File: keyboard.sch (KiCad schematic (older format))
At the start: 74 parts, among them IC1 ATMEGA32U4, J1 MINI, P1 MISO, P10 ROW4, P18 LR1, P19 LR2, P2 Vcc, P20 LR3, P200 GND, P201 GND, P202 GND, P203 GND, P21 LR4, P23 LC1, P24 LC2, P25 LC3, P26 LC4, P27 LC5, P28 LC6, P29 LC7, P3 SCK, P30 LC8, P31 LC9, P32 LC10, P33 LC11, P34 LC12, P35 LGND, P36 LVcc, P37 Vcc, P38 GPIO0, P39 GPIO1, P4 MOSI, P40 GPIO2, P41 GPIO3, P42 GPIO4(SS), P43 GPIO5(SCK), P44 GPIO6(MOSI), P45 GPIO7(SCL), P46 GPIO8(SDA), P47 GND, P5 RES, P6 GND, P7 ROW1, P8 ROW2, P9 ROW3, X1 CRYSTAL

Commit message: Rebuild the project using latest kicad
Rebuild the project using latest kicad, leaving eschematic and pcb
unfinished
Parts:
- removed C4, C5, C6, C7: 100n, symbol C
- removed C8: 1u, symbol C
- removed DF3, DW1, DW2, DW3, DW4: LED, symbol LED
- removed H1, H2, H3, H4, H5: HOLE, ~, symbol ANYTHING
- removed J1: MINI, symbol USBMINI_B05
- removed P1: MISO, symbol CONN_1
- removed P10: ROW4, symbol CONN_1
- removed P18: LR1, symbol CONN_1
- removed P19: LR2, symbol CONN_1
- removed P2, P37: Vcc, symbol CONN_1
- removed P20: LR3, symbol CONN_1
- removed P200, P201, P202, P203, P47, P6: GND, symbol CONN_1
- removed P21: LR4, symbol CONN_1
- removed P23: LC1, symbol CONN_1
- removed P24: LC2, symbol CONN_1
- removed P25: LC3, symbol CONN_1
- removed P26: LC4, symbol CONN_1
- removed P27: LC5, symbol CONN_1
- removed P28: LC6, symbol CONN_1
- removed P29: LC7, symbol CONN_1
- removed P3: SCK, symbol CONN_1
- removed P30: LC8, symbol CONN_1
- removed P31: LC9, symbol CONN_1
- removed P32: LC10, symbol CONN_1
- removed P33: LC11, symbol CONN_1
- removed P34: LC12, symbol CONN_1
- removed P35: LGND, symbol CONN_1
- removed P36: LVcc, symbol CONN_1
- removed P38: GPIO0, symbol CONN_1
- removed P39: GPIO1, symbol CONN_1
- removed P4: MOSI, symbol CONN_1
- removed P40: GPIO2, symbol CONN_1
- removed P41: GPIO3, symbol CONN_1
- removed P42: GPIO4(SS), symbol CONN_1
- removed P43: GPIO5(SCK), symbol CONN_1
- removed P44: GPIO6(MOSI), symbol CONN_1
- removed P45: GPIO7(SCL), symbol CONN_1
- removed P46: GPIO8(SDA), symbol CONN_1
- removed P5: RES, symbol CONN_1
- removed P7: ROW1, symbol CONN_1
- removed P8: ROW2, symbol CONN_1
- removed P9: ROW3, symbol CONN_1
- removed R12, RW1, RW2, RW3, RW4: R, symbol R
- removed R3: 10k, symbol R
- removed X1: CRYSTAL, symbol CRYSTAL
- added J?: USBMINI_B05, symbol USBMINI_B05
- added R?: R, symbol R
- added X?: CRYSTAL, symbol CRYSTAL
- C1, C2: value 22p -> 22pF; Product CL21C220JBANNNC -> (none); Supplier TME -> (none); Supplier Symbol CL21C220JBANNNC -> (none); Vendor Samsung -> (none)
- C3: value 1u -> 1uF; Product CL21B105KAFNNNE -> (none); Supplier TME -> (none); Supplier Symbol CL21B105KAFNNNE -> (none); Vendor Samsung -> (none)
- IC1: Product ATmega32U4-AU -> (none); Supplier DigiKey -> (none); Supplier Symbol ATMEGA32U4-AU-ND -> (none); Vendor Atmel -> (none)
- R1, R2: value 22 -> 22R; Product CRCW080522R0JNTABC -> (none); Supplier TME -> (none); Supplier Symbol CRCW080522R0JNTABC -> (none); Vendor Vishay -> (none)
- R5: value 10k -> 10K; Product CRCW080510K0JNTABC -> (none); Supplier TME -> (none); Supplier Symbol CRCW080510K0JNTABC -> (none); Vendor Vishay -> (none)
- S0: Product TACTB-64K-F -> (none); Supplier TME -> (none); Supplier Symbol TACTB-64K-F -> (none); Vendor Ninigi -> (none)
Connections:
- net labels removed: D+, D-, GPIO0, GPIO1, GPIO2, GPIO3, GPIO4, GPIO5, GPIO6, GPIO7, GPIO8, MISO, MOSI, SCK, SCL, SDA, SS, caps, col1, col10, col11, col2, col3, col4, col5, col6, col7, col8, col9, row1, row2, row3, row4, ~RES~
- wire segments 168 -> 46
- no-connect marks 4 -> 2
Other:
- note removed: "Expansion\nconnector \n(right)"
- note removed: "FN LED\n"
- note removed: "Ground Pins"
- note removed: "ISP Pins"
- note removed: "LED Matrix\n(top)"
- note removed: "Mounting\nHoles"
- note removed: "PWM"
- note removed: "SW01 LED (ESCAPE)\n"
- note removed: "WASD Cluster LEDs\n"

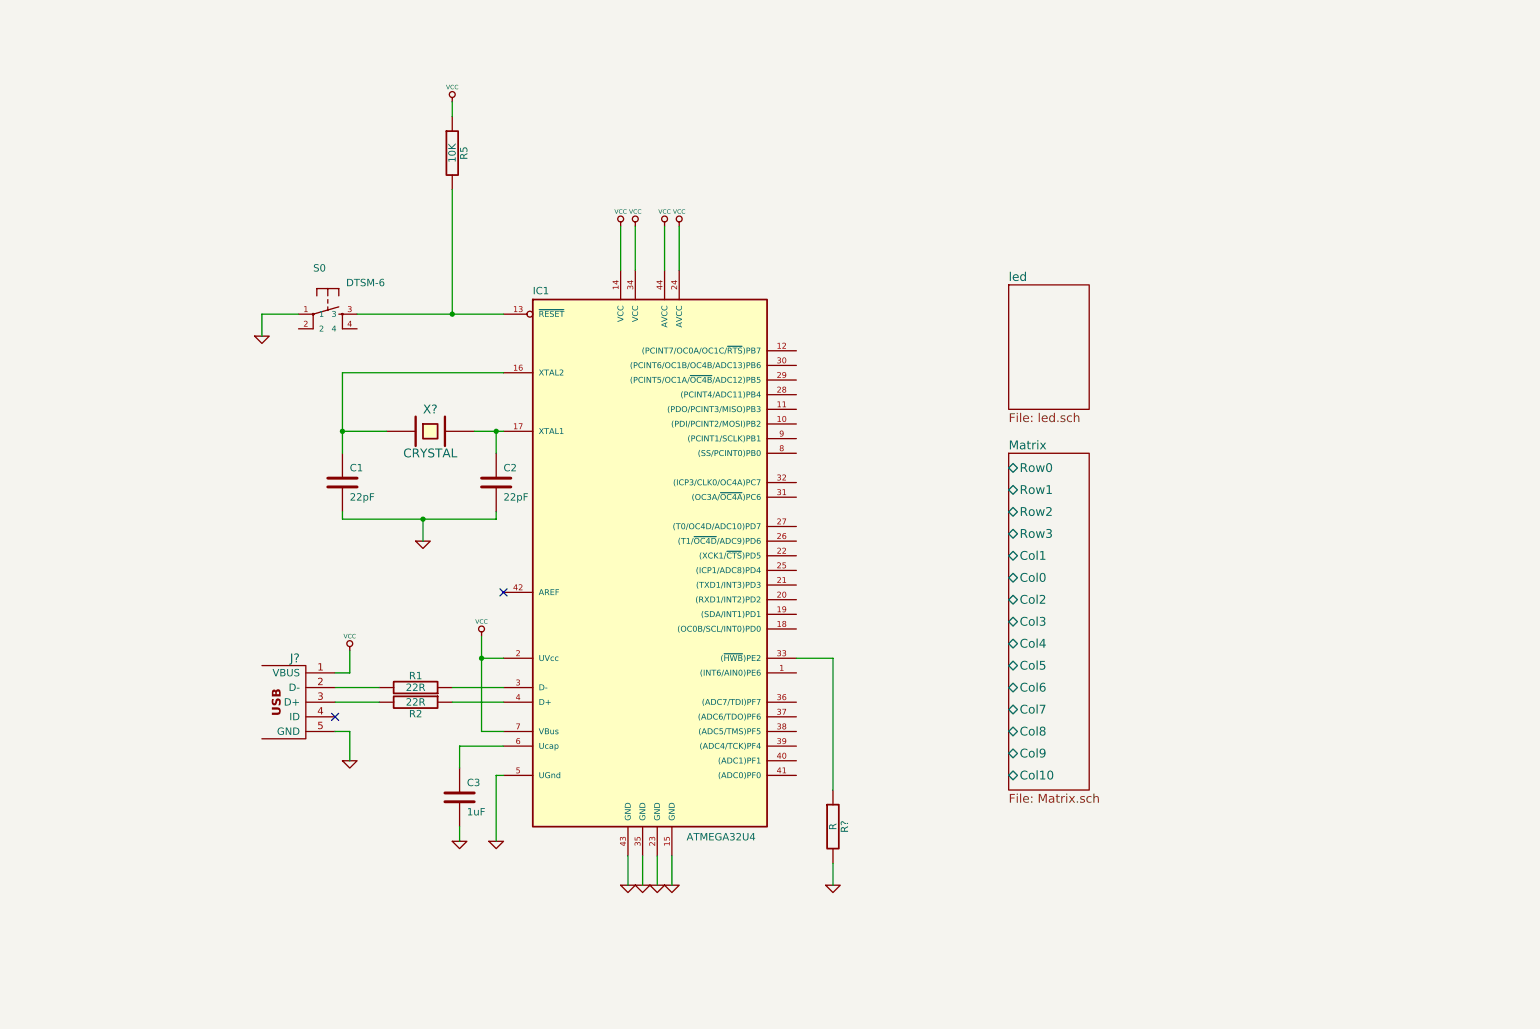
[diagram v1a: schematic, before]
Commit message: Final touches on schematic
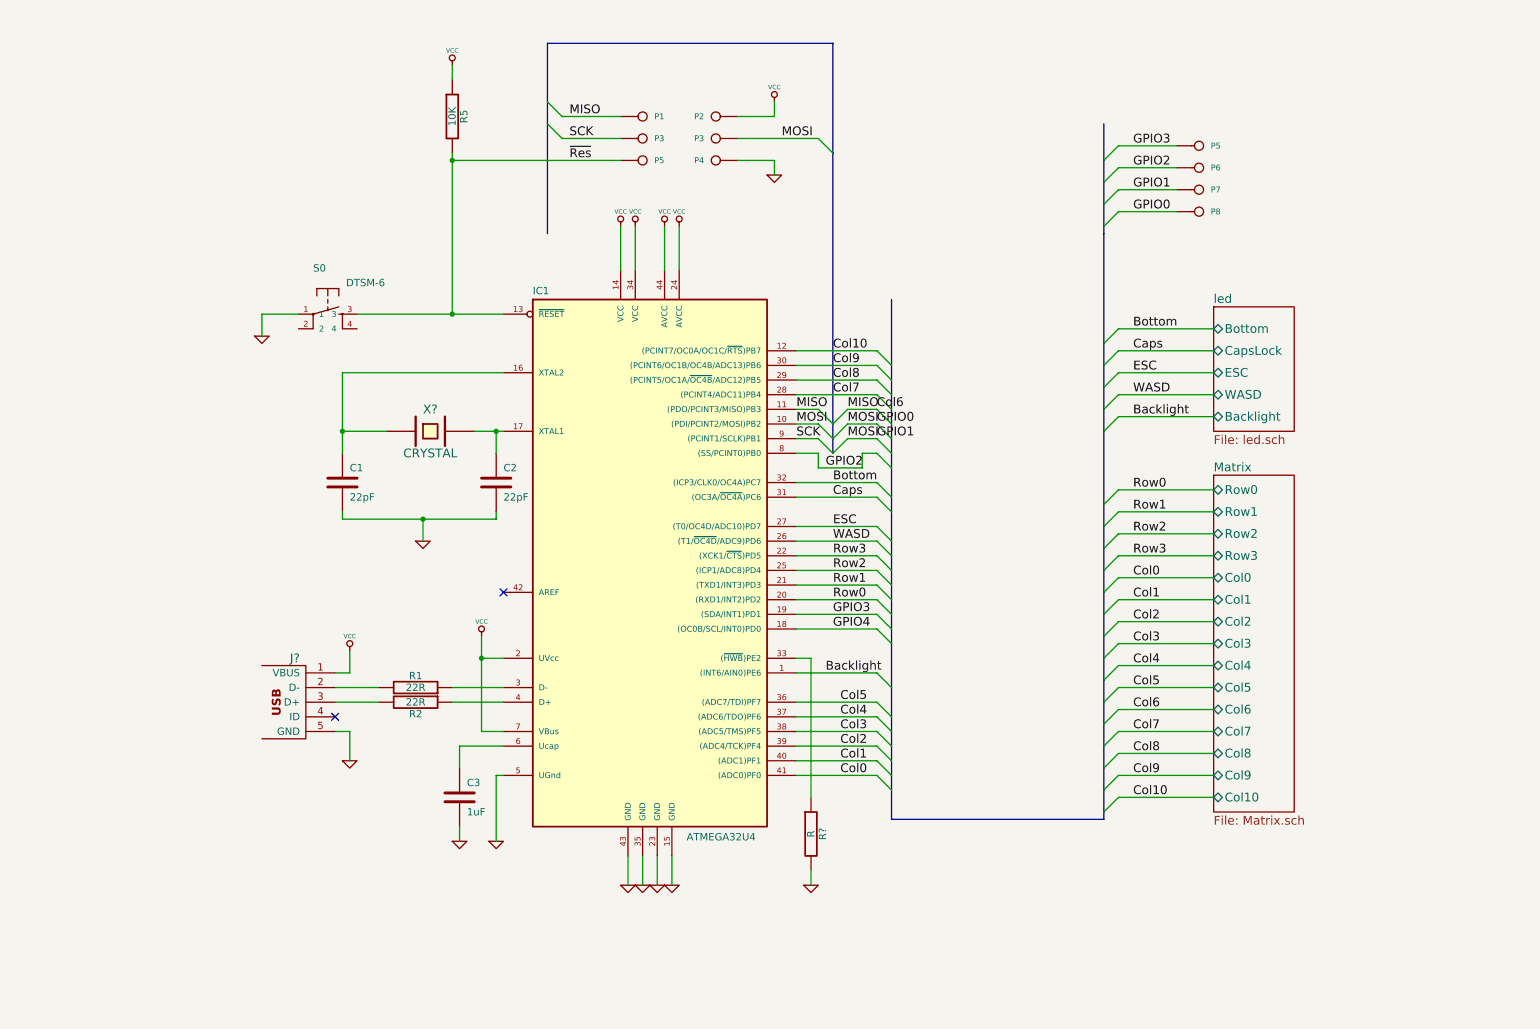
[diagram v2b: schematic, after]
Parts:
- added P1, P2, P3 (x2), P4, P5 (x2), P6, P7, P8: CONN_1, symbol CONN_1
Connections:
- net GND: now also P4.1
- net VCC: now also P2.1
- net Backlight: now reaches IC1.1 ((INT6/AIN0)PE6)
- net GPIO0: now reaches IC1.10 ((PDI/PCINT2/MOSI)PB2)
- net GPIO0: now also P3.1, P7.1, P8.1
- net Col6: now reaches IC1.11 ((PDO/PCINT3/MISO)PB3)
- net Col6: now also P1.1
- net Col10: now reaches IC1.12 ((PCINT7/OC0A/OC1C/~RTS~)PB7)
- net ~Res: now reaches IC1.13 (~RESET~), R5.2, S0.3
- net ~Res: now also P5.1
- net GPIO4: now reaches IC1.18 ((OC0B/SCL/INT0)PD0)
- net GPIO3: now reaches IC1.19 ((SDA/INT1)PD1)
- net GPIO3: now also P5.1
- net Row0: now reaches IC1.20 ((RXD1/INT2)PD2)
- net Row1: now reaches IC1.21 ((TXD1/INT3)PD3)
- net Row3: now reaches IC1.22 ((XCK1/~CTS~)PD5)
- net Row2: now reaches IC1.25 ((ICP1/ADC8)PD4)
- net WASD: now reaches IC1.26 ((T1/~OC4D~/ADC9)PD6)
- net ESC: now reaches IC1.27 ((T0/OC4D/ADC10)PD7)
- net Col7: now reaches IC1.28 ((PCINT4/ADC11)PB4)
- net Col8: now reaches IC1.29 ((PCINT5/OC1A/~OC4B~/ADC12)PB5)
- net Col9: now reaches IC1.30 ((PCINT6/OC1B/OC4B/ADC13)PB6)
- net Caps: now reaches IC1.31 ((OC3A/~OC4A~)PC6)
- net Bottom: now reaches IC1.32 ((ICP3/CLK0/OC4A)PC7)
- net Col5: now reaches IC1.36 ((ADC7/TDI)PF7)
- net Col4: now reaches IC1.37 ((ADC6/TDO)PF6)
- net Col3: now reaches IC1.38 ((ADC5/TMS)PF5)
- net Col2: now reaches IC1.39 ((ADC4/TCK)PF4)
- net Col1: now reaches IC1.40 ((ADC1)PF1)
- net Col0: now reaches IC1.41 ((ADC0)PF0)
- net GPIO2: now reaches IC1.8 ((SS/PCINT0)PB0)
- net GPIO2: now also P6.1
- net SCK: now reaches IC1.9 ((PCINT1/SCLK)PB1)
- net SCK: now also P3.1
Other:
- moved on the sheet: R5, R?
